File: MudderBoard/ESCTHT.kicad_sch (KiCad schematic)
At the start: 82 parts, among them M3 N-MOSFET, M4 N-MOSFET, U8 LM5122QMH/NOPB, U9 LM5122QMH/NOPB

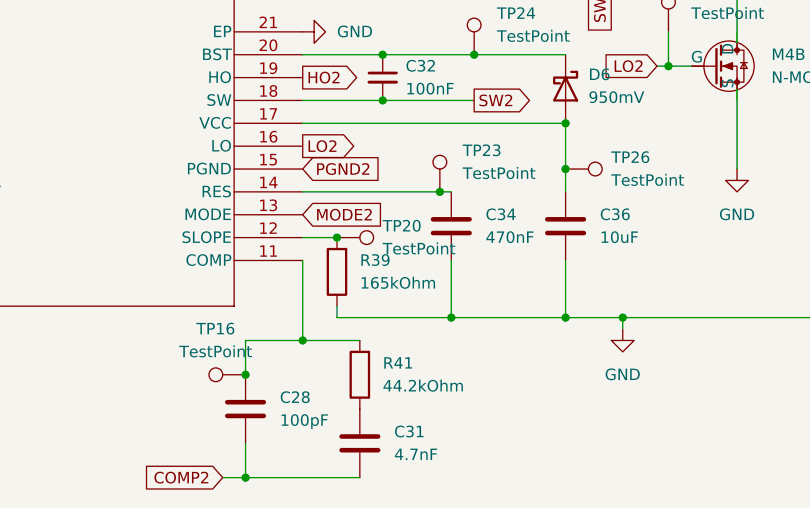
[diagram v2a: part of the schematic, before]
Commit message: revert to colin changes
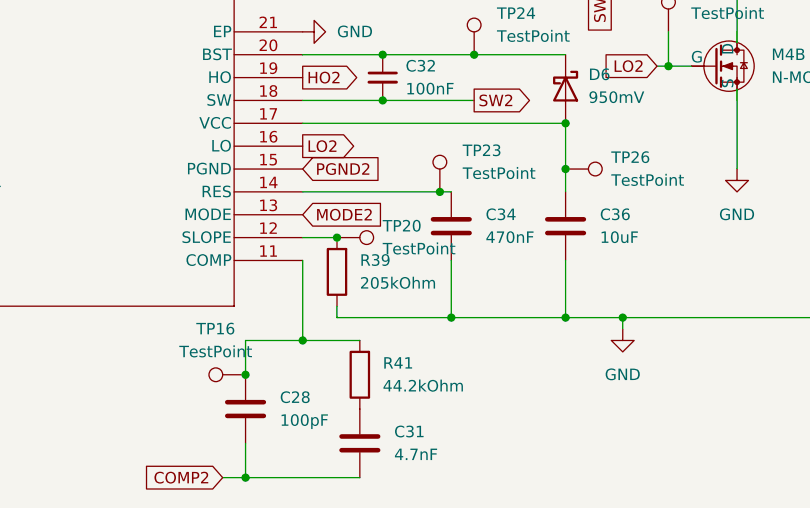
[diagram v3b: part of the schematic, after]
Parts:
- R39: value 165kOhm -> 205kOhm
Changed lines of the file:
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@@
 	)
 	(junction
+		(at 176.53 137.16)
+		(diameter 0)
+		(color 0 0 0 0)
+	)
+	(junction
 		(at 240.03 100.33)
 		(diameter 0)
@@
 	)
 	(junction
-		(at 176.53 137.16)
-		(diameter 0)
-		(color 0 0 0 0)
-	)
-	(junction
 		(at 248.92 26.67)
 		(diameter 0)
@@
 	)
 	(symbol
-		(lib_id "Device:R")
-		(at 176.53 140.97 180)
-		(unit 1)
-		(exclude_from_sim no)
-		(in_bom yes)
-		(on_board yes)
-		(dnp no)
-		(fields_autoplaced yes)
-		(property "Reference" "R39"
-			(at 179.07 139.6999 0)
-			(effects
-				(font
-					(size 1.27 1.27)
-				)
-				(justify right)
-			)
-		)
-		(property "Value" "165kOhm"
-			(at 179.07 142.2399 0)
-			(effects
-				(font
-					(size 1.27 1.27)
-				)
-				(justify right)
-			)
-		)
-		(property "Footprint" "Lidar_Foot:RESC1005X40N"
-			(at 178.308 140.97 90)
-			(effects
-				(font
-					(size 1.27 1.27)
-				)
-				(hide yes)
-			)
-		)
-		(property "Datasheet" "~"
-			(at 176.53 140.97 0)
-			(effects
-				(font
-					(size 1.27 1.27)
-				)
-				(hide yes)
-			)
-		)
-		(property "Description" "Resistor"
-			(at 176.53 140.97 0)
-			(effects
-				(font
-					(size 1.27 1.27)
-				)
-				(hide yes)
-			)
-		)
-		(pin "1"
-		)
-		(pin "2"
-		)
-		(instances
-			(project "MudderBoard"
-				(path "/cdf98bf7-80ce-4b13-b655-e6c7c589c122/156878a8-0263-42d4-a037-3f42ee3dc0ef"
-					(reference "R39")
-					(unit 1)
-				)
-			)
-		)
-	)
-	(symbol
 		(lib_id "Connector:TestPoint")
 		(at 58.42 128.27 90)
@@
 					(unit 1)
 				)
+			)
+		)
+	)
+	(symbol
+		(lib_id "Device:R")
+		(at 176.53 140.97 180)
+		(unit 1)
+		(exclude_from_sim no)
+		(in_bom yes)
+		(on_board yes)
+		(dnp no)
+		(fields_autoplaced yes)
+		(property "Reference" "R39"
+			(at 179.07 139.6999 0)
+			(effects
+				(font
+					(size 1.27 1.27)
+				)
+				(justify right)
+			)
+		)
+		(property "Value" "205kOhm"
+			(at 179.07 142.2399 0)
+			(effects
+				(font
+					(size 1.27 1.27)
+				)
+				(justify right)
+			)
+		)
+		(property "Footprint" "Lidar_Foot:RESC1005X40N"
+			(at 178.308 140.97 90)
+			(effects
+				(font
+					(size 1.27 1.27)
+				)
+				(hide yes)
+			)
+		)
+		(property "Datasheet" "~"
+			(at 176.53 140.97 0)
+			(effects
+				(font
+					(size 1.27 1.27)
+				)
+				(hide yes)
+			)
+		)
+		(property "Description" "Resistor"
+			(at 176.53 140.97 0)
+			(effects
+				(font
+					(size 1.27 1.27)
+				)
+				(hide yes)
+			)
+		)
+		(pin "1"
+		)
+		(pin "2"
+		)
+		(instances
+			(project "MudderBoard"
+				(path "/cdf98bf7-80ce-4b13-b655-e6c7c589c122/156878a8-0263-42d4-a037-3f42ee3dc0ef"
+					(reference "R39")
+					(unit 1)
+				)
